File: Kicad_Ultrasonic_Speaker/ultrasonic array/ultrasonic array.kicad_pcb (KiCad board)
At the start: 2 copper layers, 111.3 x 93 mm, 37 parts, among them J1 Screw_Terminal_01x02_from_cir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

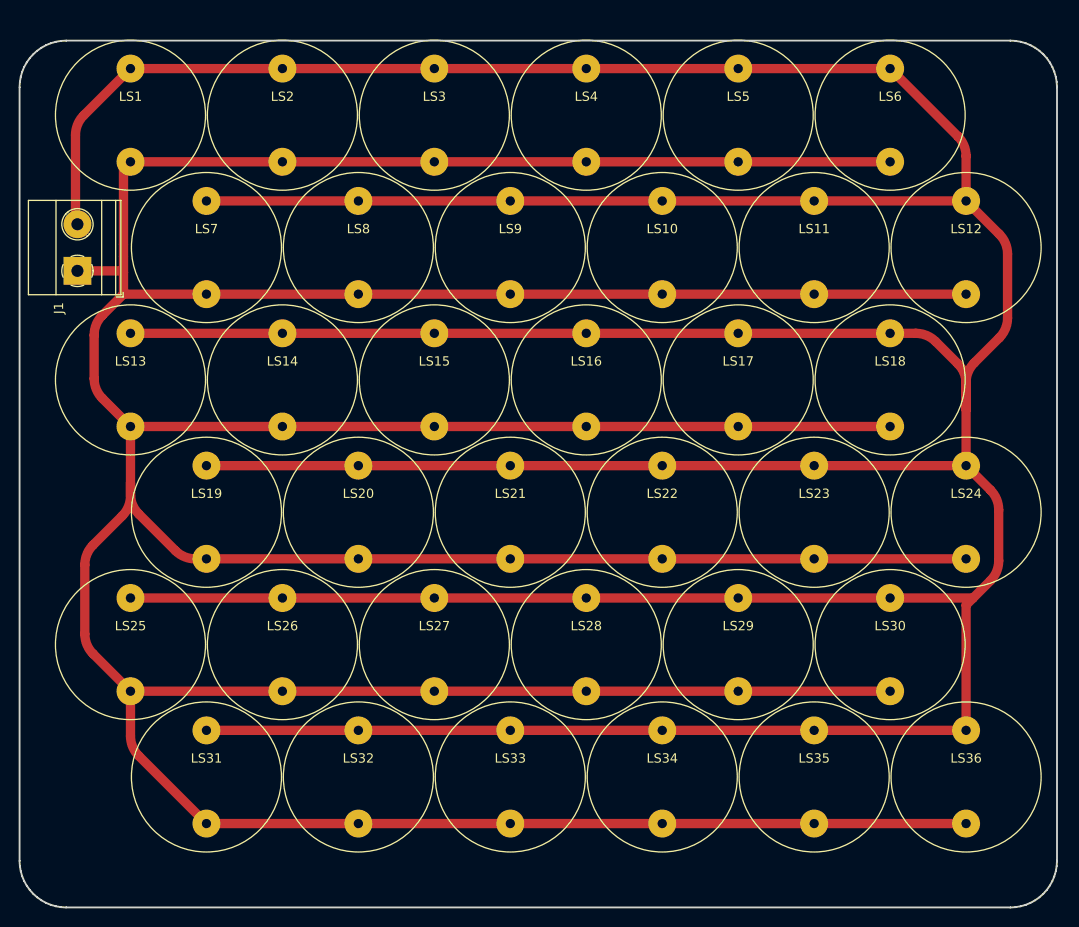
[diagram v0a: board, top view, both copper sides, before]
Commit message: change kicad
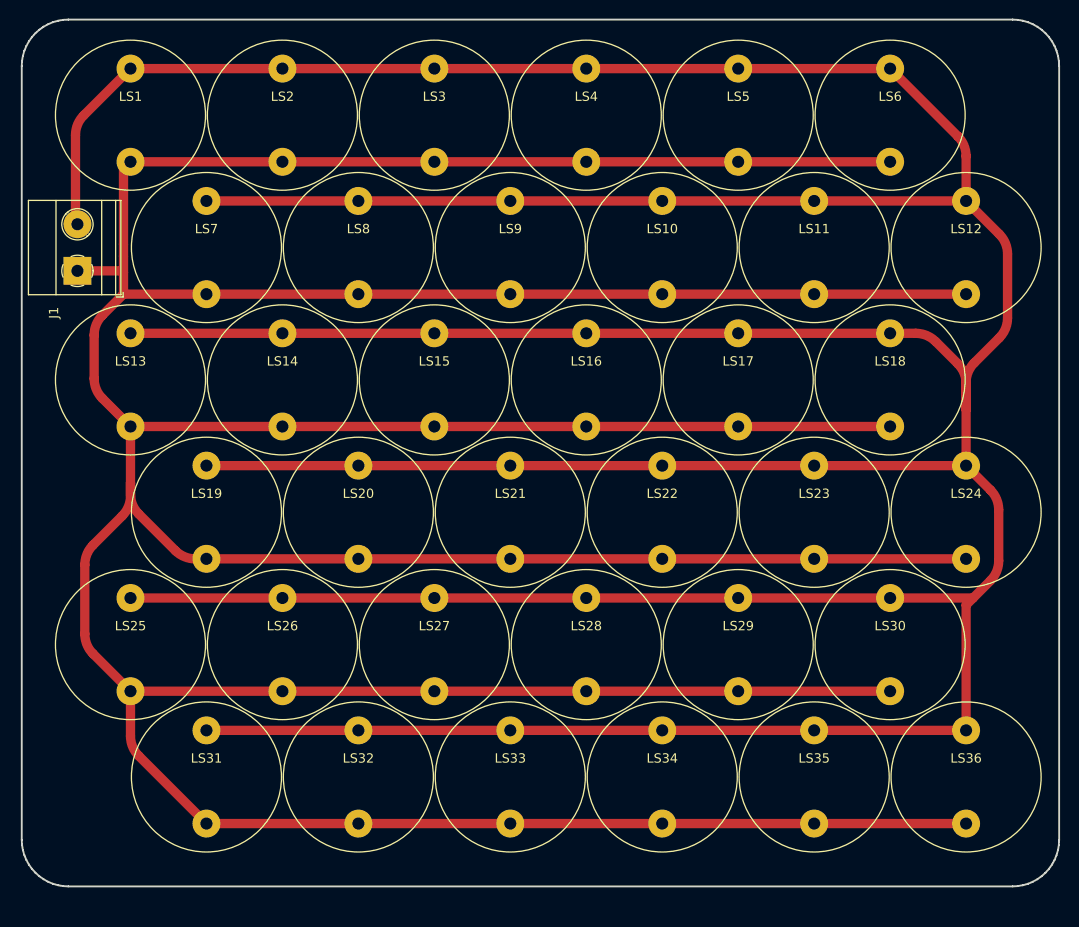
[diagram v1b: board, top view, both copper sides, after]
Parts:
- J1: value Screw_Terminal_01x02_from_circuit -> Screw_Terminal_01x02
